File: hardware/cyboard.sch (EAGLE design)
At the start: 31 parts, among them CON1 CPCBUS, IC1 PIC16F84AP, IC2 74HCT21N, IC3 74HCT244N, IC4 GAL20V8B, IC5 DS12887A

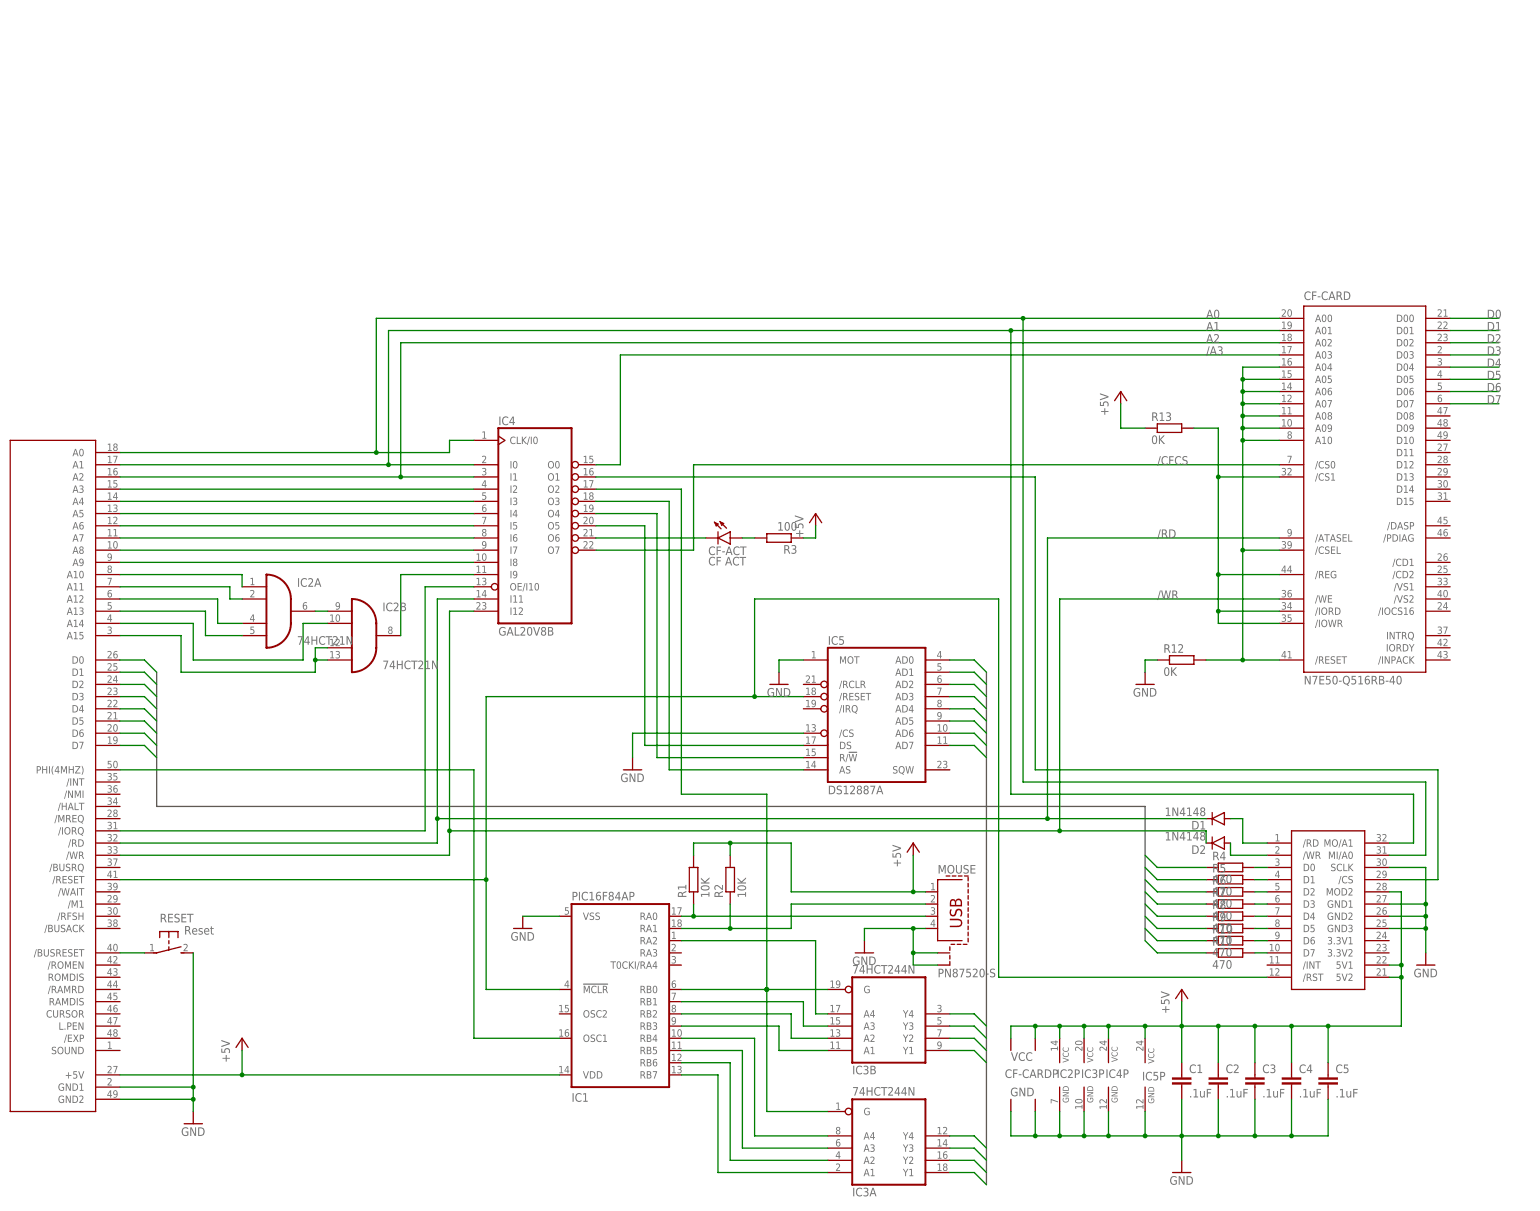
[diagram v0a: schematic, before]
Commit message: Add files via upload
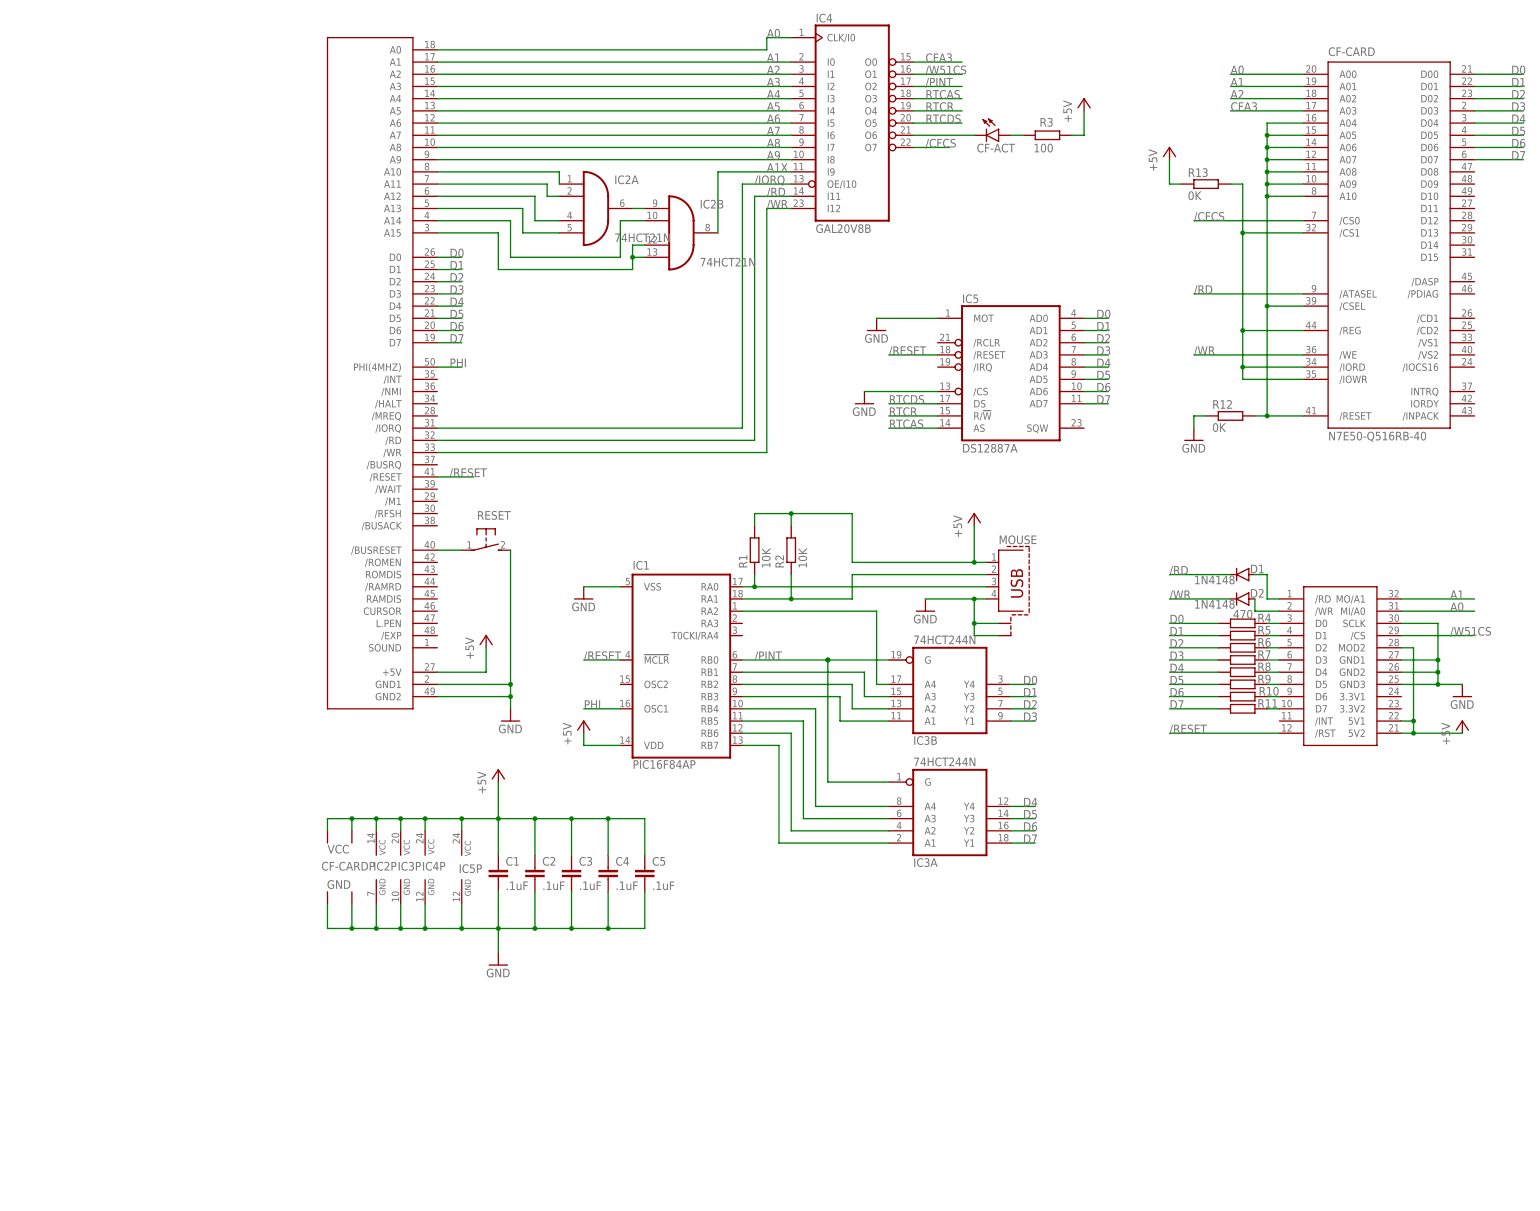
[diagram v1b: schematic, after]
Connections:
- net /A3 renamed CFA3
- net /MOUSEINT renamed /PINT
- net ADDR1015 renamed A1X
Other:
- moved on the sheet: C1, C2, C3, C4, C5, CF-ACT, CF-CARD, CF-CARDP, D1, D2, IC1, IC2A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
